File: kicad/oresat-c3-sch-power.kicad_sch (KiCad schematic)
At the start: 58 parts, among them U31 LP2985AIM5-3.3, U34 TPS259621DDA, U35 TPS259620DDA, U36 LTC3624-5, U38 LP2985AIM5-3.3, U6 LTC3624-5

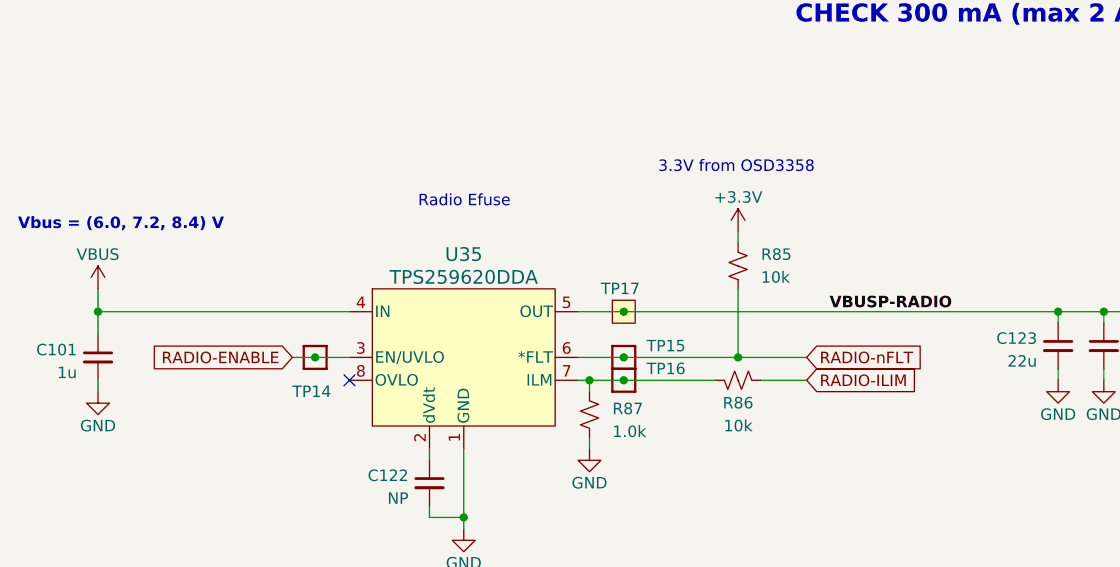
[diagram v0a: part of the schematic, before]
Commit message: Zero airwires! Rough draft schematic and layout are done. Still need ERC and DRC and full design review and stiching and polish.
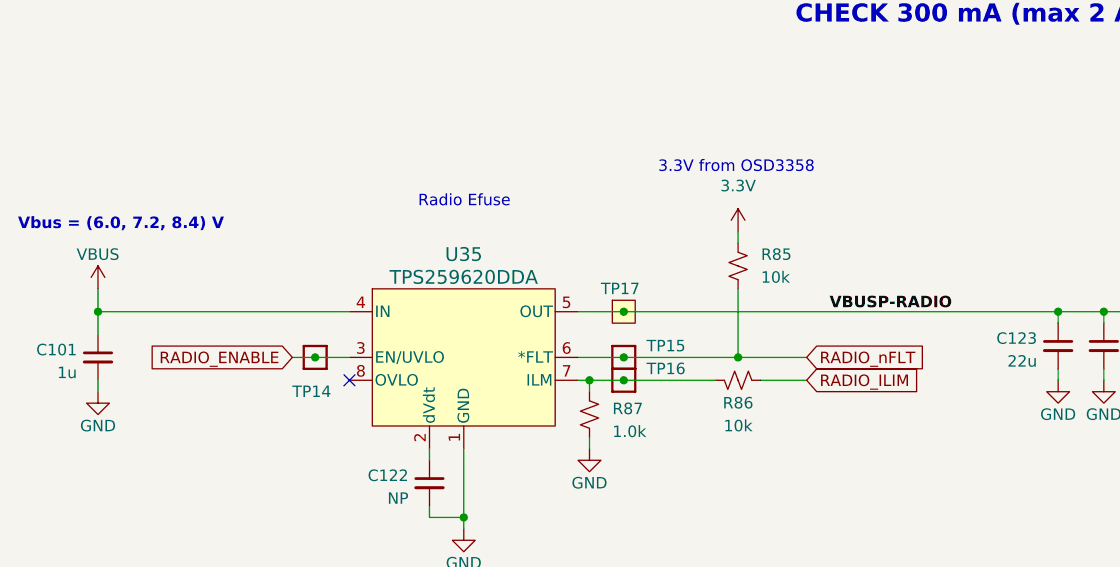
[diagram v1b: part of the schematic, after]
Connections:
- net +3.3V renamed 3.3V
- net RADIO-ENABLE renamed RADIO_ENABLE
- net RADIO-ILIM renamed RADIO_ILIM
- net RADIO-nFLT renamed RADIO_nFLT
